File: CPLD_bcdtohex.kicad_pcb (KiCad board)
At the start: 2 copper layers, 25 parts, among them IC1 ATF750C-10PU, SW1 SW_DIP_x06

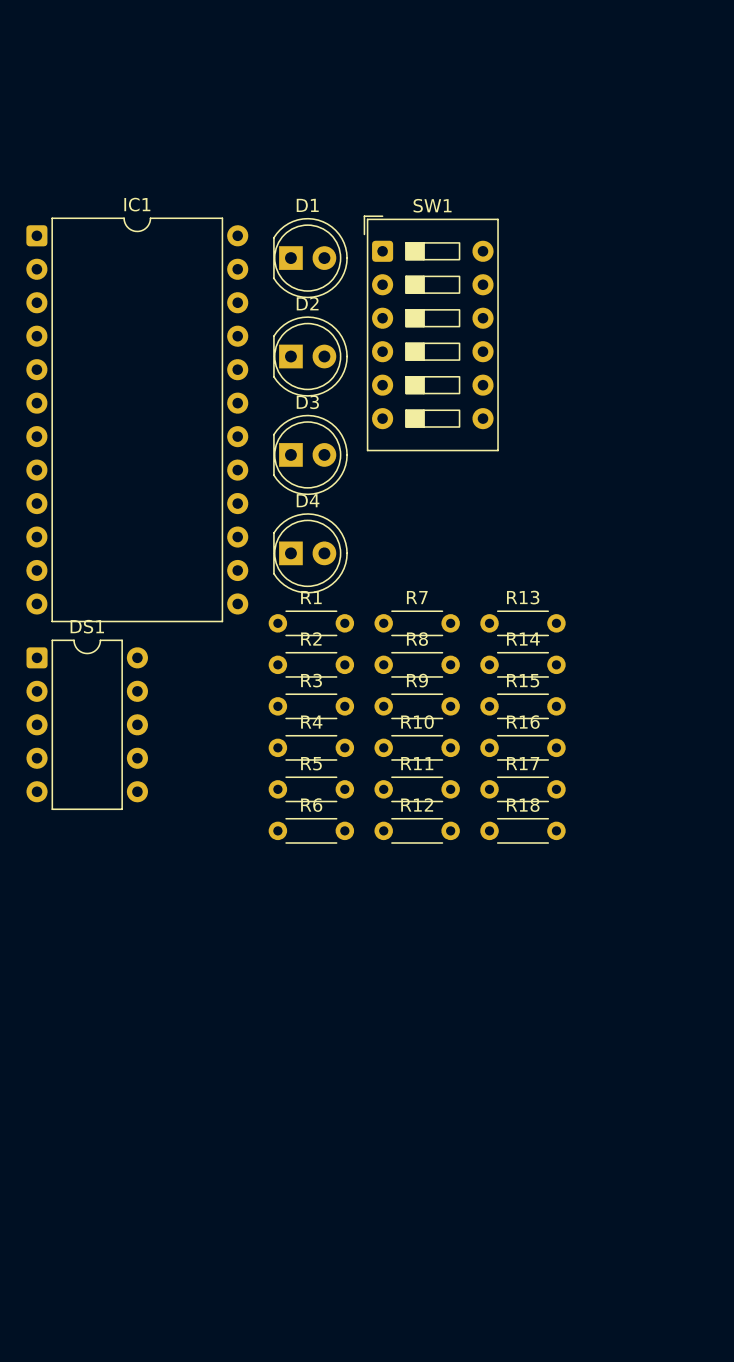
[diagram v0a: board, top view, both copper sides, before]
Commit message: Initial commit
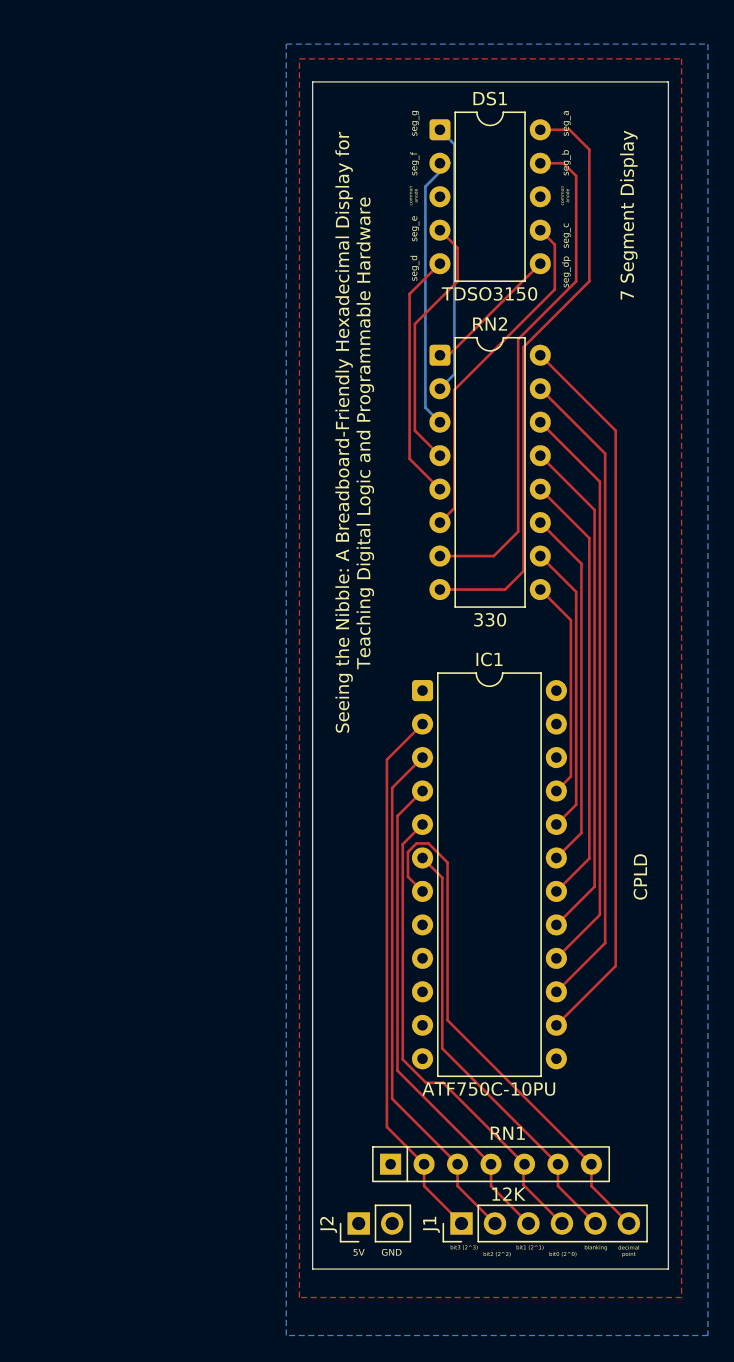
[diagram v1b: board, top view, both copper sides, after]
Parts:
- removed D1, D2, D3, D4: LED, LED_THT:LED_D5.0mm
- removed R1, R2, R3, R4, R5, R6: 10k, Resistor_THT:R_Axial_DIN0204_L3.6mm_D1.6mm_P5.08mm_Horizontal
- removed R10, R11, R12, R13, R14, R7, R8, R9: 330, Resistor_THT:R_Axial_DIN0204_L3.6mm_D1.6mm_P5.08mm_Horizontal
- removed R15, R16, R17, R18: 220, Resistor_THT:R_Axial_DIN0204_L3.6mm_D1.6mm_P5.08mm_Horizontal
- removed SW1: SW_DIP_x06, Button_Switch_THT:SW_DIP_SPSTx06_Slide_9.78x17.42mm_W7.62mm_P2.54mm
- added J1: Conn_01x06, Connector_PinHeader_2.54mm:PinHeader_1x06_P2.54mm_Vertical, F.Cu at (150.3, 148.5)
- added J2: Conn_01x02, Connector_PinHeader_2.54mm:PinHeader_1x02_P2.54mm_Vertical, F.Cu at (142.5, 148.5)
- added RN1: 12K, Resistor_THT:R_Array_SIP7, F.Cu at (144.9, 144.0)
- added RN2: 330, Package_DIP:DIP-16_W7.62mm, F.Cu at (148.7, 82.6)
- IC1: footprint Package_DIP:DIP-24_W15.24mm -> Package_DIP:DIP-24_W10.16mm
- moved DS1 50.4 mm to (148.7, 65.5)
- moved IC1 45.3 mm to (147.3, 108.1)
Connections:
- DS1 pad 1: Net-(DS1-g) -> /g
- DS1 pad 10: Net-(DS1-a) -> /a
- DS1 pad 2: Net-(DS1-f) -> /f
- DS1 pad 4: Net-(DS1-e) -> /e
- DS1 pad 5: Net-(DS1-d) -> /d
- DS1 pad 6: Net-(DS1-DP) -> /dp
- DS1 pad 7: Net-(DS1-c) -> /c
- DS1 pad 9: Net-(DS1-b) -> /b
- IC1 pad 2: Net-(IC1-IN_1) -> /bit3_in
- IC1 pad 3: Net-(IC1-IN_2) -> /bit2_in
- IC1 pad 4: Net-(IC1-IN_3) -> /bit1_in
- IC1 pad 5: Net-(IC1-IN_4) -> /bit0_in
- IC1 pad 6: Net-(IC1-IN_5) -> /BLANK_in
- IC1 pad 7: Net-(IC1-IN_6) -> /DP_in
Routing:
- net Net-(IC1-I/O_1): track 0.00 -> 55.1 mm
- net Net-(IC1-I/O_2): track 0.00 -> 49.3 mm
- net /a: track 0.00 -> 45.3 mm
- net Net-(IC1-I/O_3): track 0.00 -> 43.9 mm
- net /bit3_in: track 0.00 -> 41.4 mm
- net /DP_in: track 0.00 -> 40.4 mm
- net /bit2_in: track 0.00 -> 39.5 mm
- net /b: track 0.00 -> 38.6 mm
- net Net-(IC1-I/O_4): track 0.00 -> 38.5 mm
- net /bit1_in: track 0.00 -> 37.7 mm
- net /bit0_in: track 0.00 -> 36.8 mm
- net /BLANK_in: track 0.00 -> 33.2 mm
- net Net-(IC1-I/O_5): track 0.00 -> 33.1 mm
- net Net-(IC1-I/O_6): track 0.00 -> 27.5 mm
- net /c: track 0.00 -> 26.3 mm
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- added copper zone on F.Cu, net +5V
- added copper zone on B.Cu, net GND
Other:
- board outline added: 27 x 90.1 mm
- board text added: "5V"
- board text added: "7 Segment Display"
- board text added: "CPLD"
- board text added: "GND"
- board text added: "Seeing the Nibble: A Breadboard-Friendly Hexadecimal Display for Teaching Digital Logic and Programmable Hardware"
- board text added: "bit0 (2^0)"
- board text added: "bit1 (2^1)"
- board text added: "bit2 (2^2)"
- board text added: "bit3 (2^3)"
- board text added: "blanking"
- board text added: "common anode"
- board text added: "decimal point"
- board text added: "seg_a"
- board text added: "seg_b"
- board text added: "seg_c"
- board text added: "seg_d"
- board text added: "seg_dp"
- board text added: "seg_e"
- board text added: "seg_f"
- board text added: "seg_g"
